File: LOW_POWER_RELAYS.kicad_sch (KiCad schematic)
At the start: 2 parts, among them CN1 6437288-3, U1 YQ506-S-112 DM

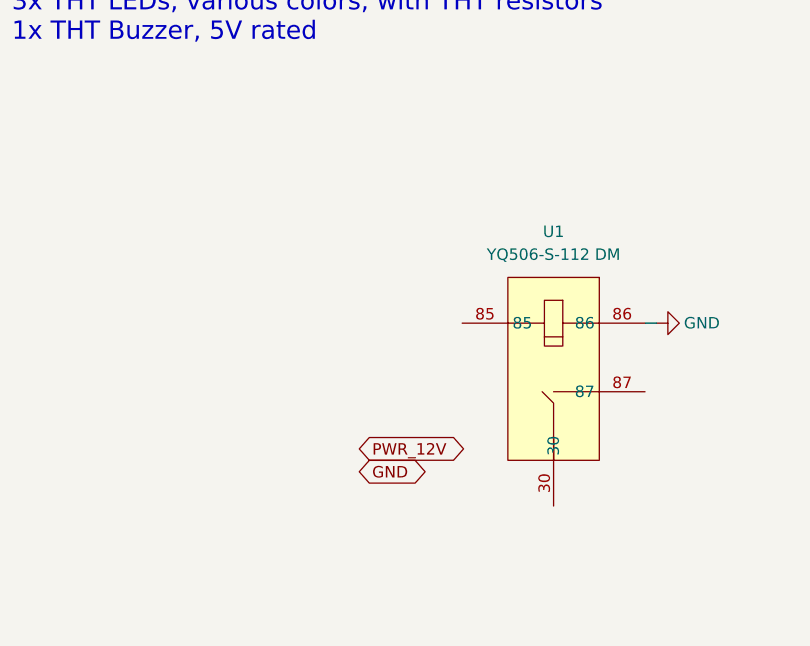
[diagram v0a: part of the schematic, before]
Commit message: Autosave
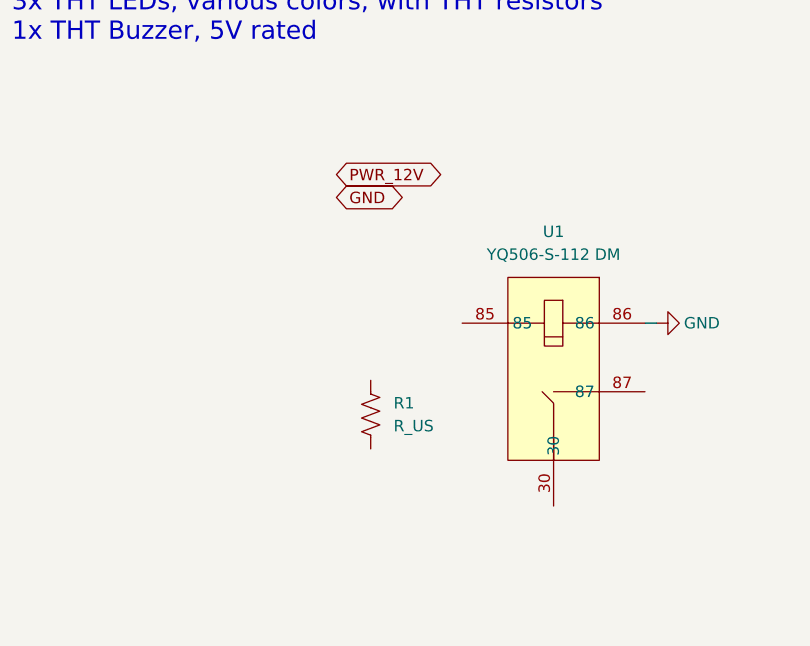
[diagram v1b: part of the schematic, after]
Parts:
- added R1: R_US, symbol Device:R_US
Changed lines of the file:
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@@
 	(global_label "GND"
 		(shape bidirectional)
-		(at 71.12 87.63 0)
+		(at 68.58 57.15 0)
 		(fields_autoplaced yes)
 		(effects
@@
 		)
 		(property "Intersheetrefs" "${INTERSHEET_REFS}"
-			(at 79.0004 87.63 0)
+			(at 76.4604 57.15 0)
 			(hide yes)
 			(show_name no)
@@
 	(global_label "PWR_12V"
 		(shape bidirectional)
-		(at 71.12 85.09 0)
+		(at 68.58 54.61 0)
 		(fields_autoplaced yes)
 		(effects
@@
 		)
 		(property "Intersheetrefs" "${INTERSHEET_REFS}"
-			(at 83.0949 85.09 0)
+			(at 80.5549 54.61 0)
 			(hide yes)
 			(show_name no)
@@
 					(unit 1)
 				)
+			)
+		)
+	)
+	(symbol
+		(lib_id "Device:R_US")
+		(at 72.39 81.28 0)
+		(unit 1)
+		(body_style 1)
+		(exclude_from_sim no)
+		(in_bom yes)
+		(on_board yes)
+		(in_pos_files yes)
+		(dnp no)
+		(fields_autoplaced yes)
+		(property "Reference" "R1"
+			(at 74.93 80.01 0)
+			(show_name no)
+			(do_not_autoplace no)
+			(effects
+				(font
+					(size 1.27 1.27)
+				)
+				(justify left)
+			)
+		)
+		(property "Value" "R_US"
+			(at 74.93 82.55 0)
+			(show_name no)
+			(do_not_autoplace no)
+			(effects
+				(font
+					(size 1.27 1.27)
+				)
+				(justify left)
+			)
+		)
+		(property "Footprint" ""
+			(at 73.406 81.534 90)
+			(hide yes)
+			(show_name no)
+			(do_not_autoplace no)
+			(effects
+				(font
+					(size 1.27 1.27)
+				)
+			)
+		)
+		(property "Datasheet" ""
+			(at 72.39 81.28 0)
+			(hide yes)
+			(show_name no)
+			(do_not_autoplace no)
+			(effects
+				(font
+					(size 1.27 1.27)
+				)
+			)
+		)
+		(property "Description" "Resistor, US symbol"
+			(at 72.39 81.28 0)
+			(hide yes)
+			(show_name no)
+			(do_not_autoplace no)
+			(effects
+				(font
+					(size 1.27 1.27)
+				)
+			)
+		)
+		(pin "1"
+		)
+		(pin "2"
+		)
+		(instances
+			(project "Hub-2.0"
+				(path "/af8ad92e-80c5-47c7-b528-865d82af0364/aea3bb0d-f9cd-46ce-9a77-d662b5a61299"
+					(reference "R1")
+					(unit 1)
+				)

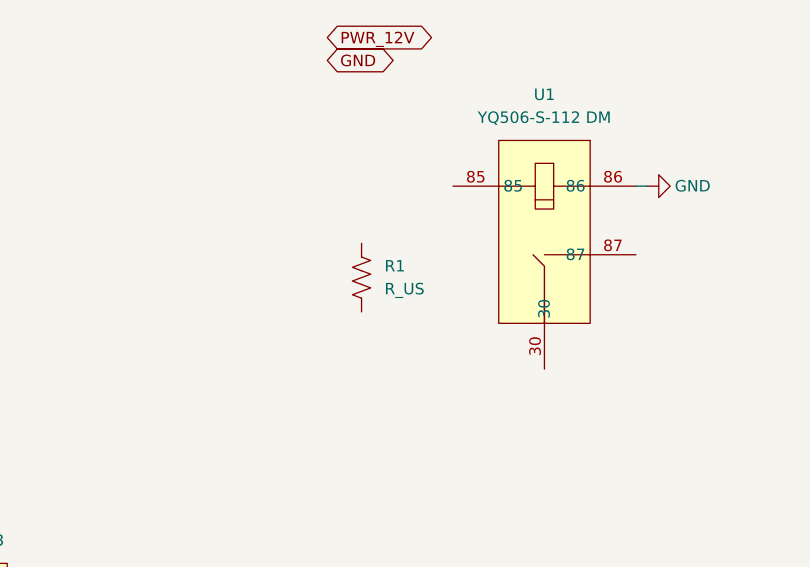
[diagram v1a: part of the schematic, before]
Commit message: Autosave
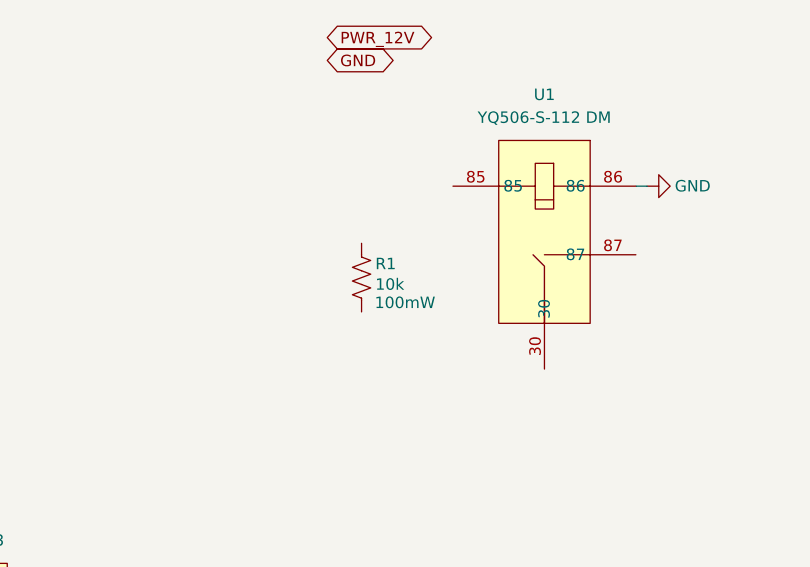
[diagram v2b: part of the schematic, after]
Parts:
- R1: value R_US -> 10k; Wattage (none) -> 100mW
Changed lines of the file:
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@@
 		(in_pos_files yes)
 		(dnp no)
-		(fields_autoplaced yes)
 		(property "Reference" "R1"
-			(at 74.93 80.01 0)
+			(at 73.914 79.756 0)
 			(show_name no)
 			(do_not_autoplace no)
@@
 			)
 		)
-		(property "Value" "R_US"
-			(at 74.93 82.55 0)
+		(property "Value" "10k"
+			(at 73.914 82.042 0)
 			(show_name no)
 			(do_not_autoplace no)
@@
 			(show_name no)
 			(do_not_autoplace no)
+			(effects
+				(font
+					(size 1.27 1.27)
+				)
+			)
+		)
+		(property "Wattage" "100mW"
+			(at 77.216 84.074 0)
+			(show_name no)
+			(do_not_autoplace no)
